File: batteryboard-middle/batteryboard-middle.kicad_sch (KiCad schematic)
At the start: 10 parts, among them J1 Conn_01x02, J2 Conn_01x02, J3 FLE-110-01-G-DV-A, J4 FLE-110-01-G-DV-A, J5 FTS-110-01-L-DV-A, J6 FTS-110-01-L-DV-A

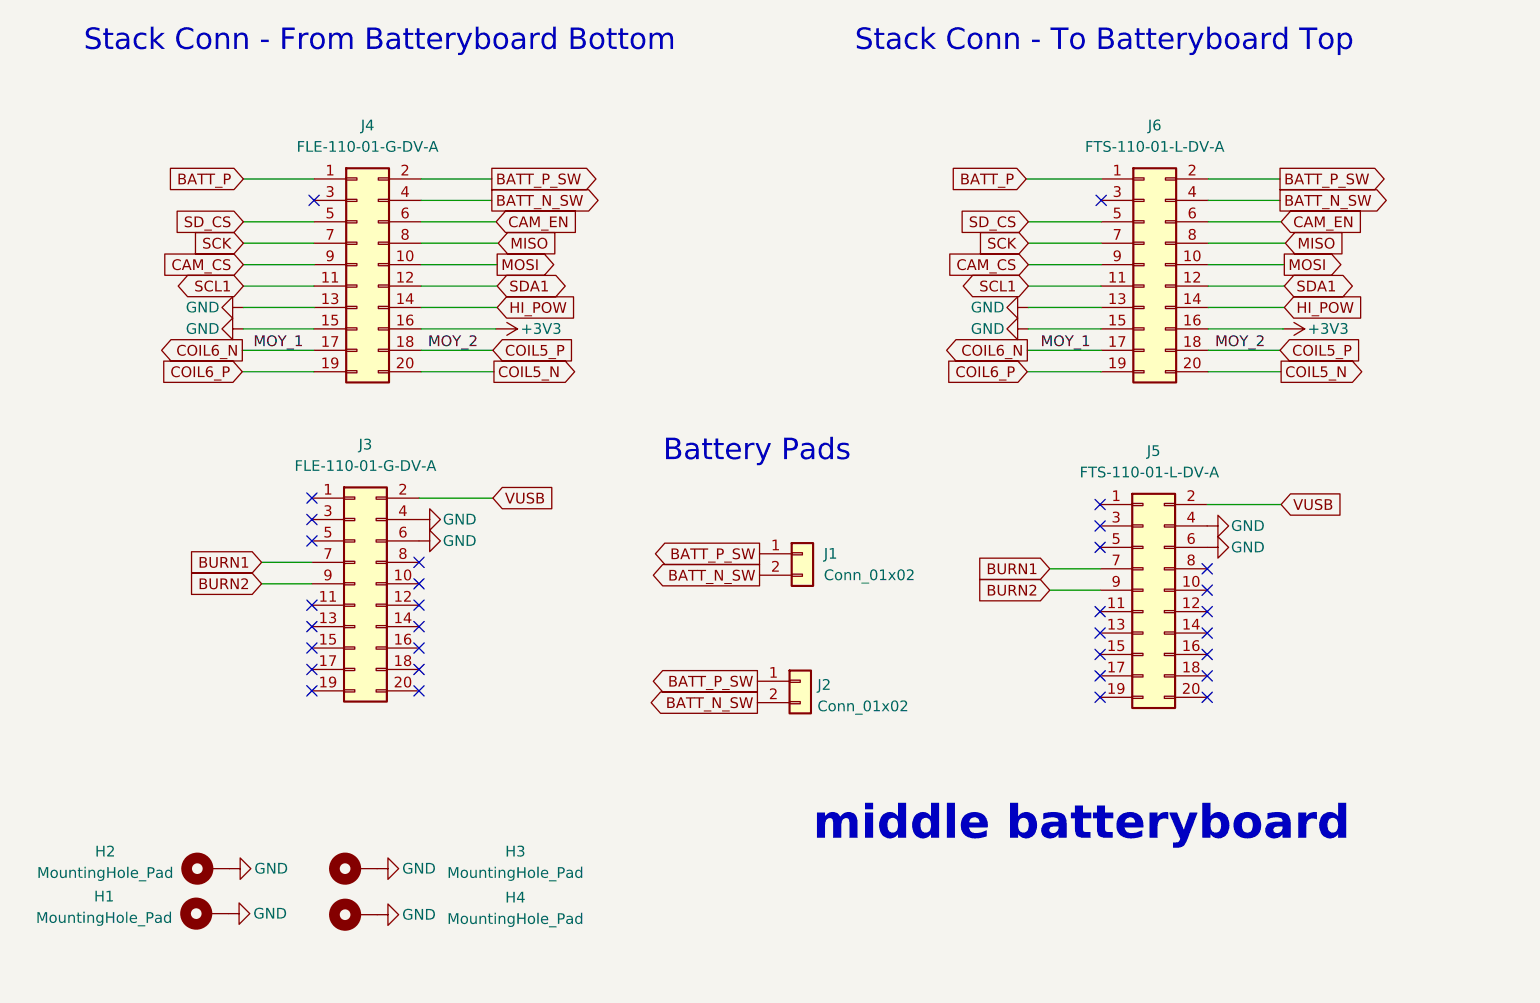
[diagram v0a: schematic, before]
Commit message: Fixed Broken Merge
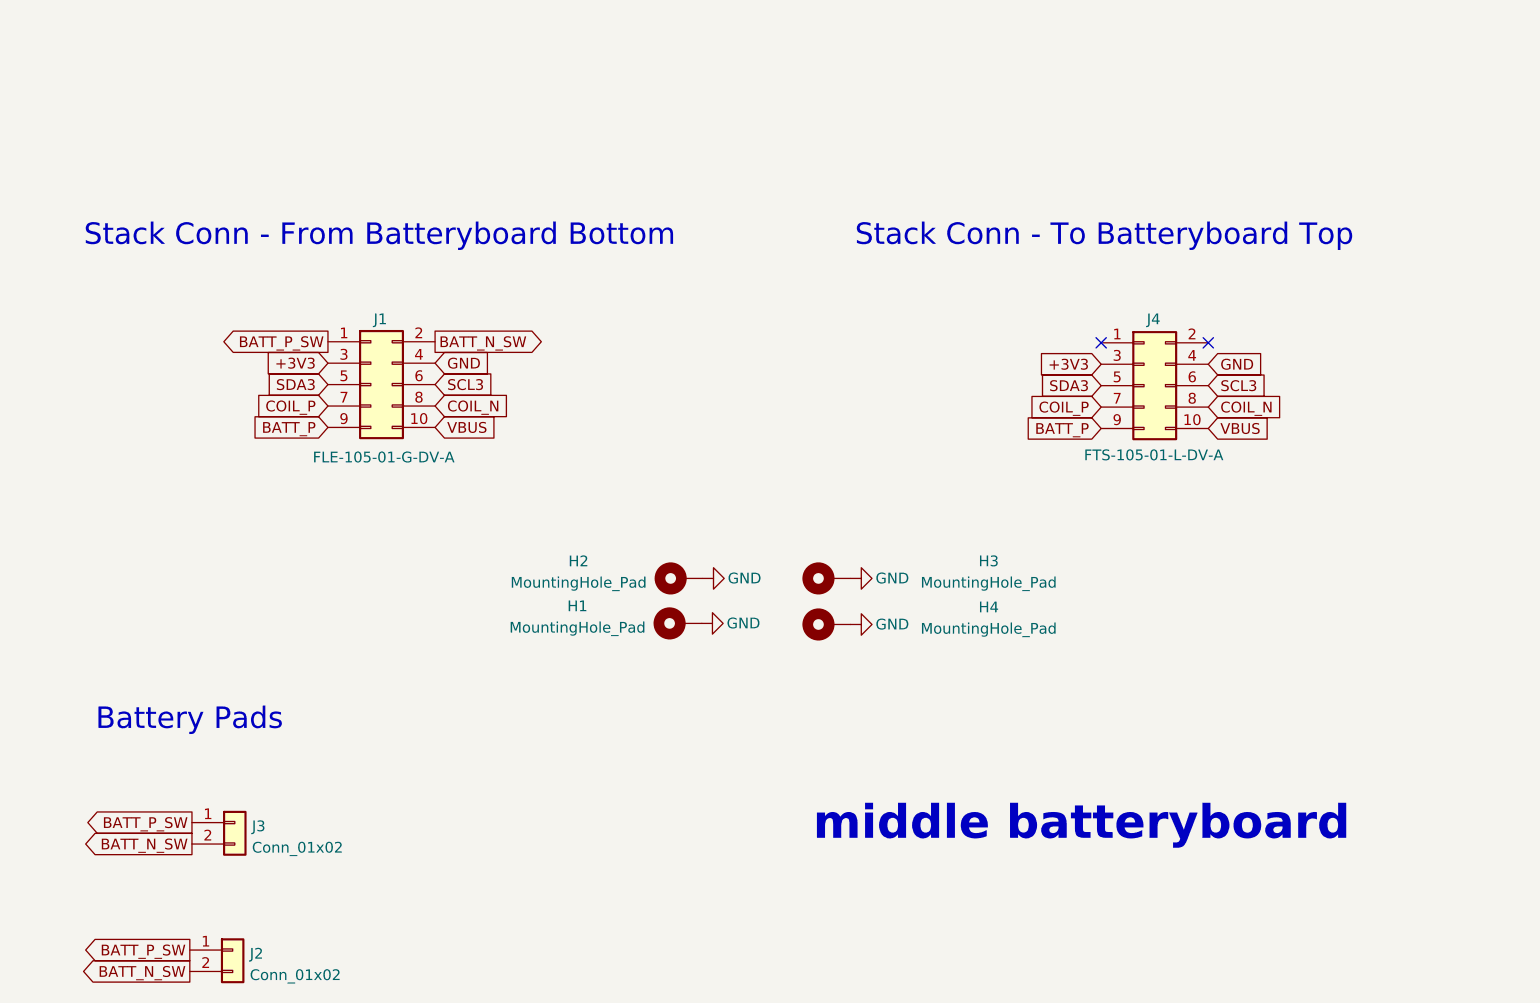
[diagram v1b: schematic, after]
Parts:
- removed J3, J4: FLE-110-01-G-DV-A, mainboard:SAMTEC_FLE-110-01-G-DV-A, symbol Connector_Generic:Conn_02x10_Odd_Even
- removed J5, J6: FTS-110-01-L-DV-A, batteryboard:SAMTEC-FTS-110-01-X-DV-A, symbol Connector_Generic:Conn_02x10_Odd_Even
- added J1: FLE-105-01-G-DV-A, batteryboard:SAMTEC_FLE-105-01-G-DV-A, symbol Connector_Generic:Conn_02x05_Odd_Even
- added J4: FTS-105-01-L-DV-A, batteryboard:FTS-105-XX-YY-DV-A, symbol Connector_Generic:Conn_02x05_Odd_Even
- renumbered J1 to J3
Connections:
- net +3V3: now also J1.3 (Pin_3), J4.3 (Pin_3)
- net BATT_N_SW: now also J1.2 (Pin_2)
- net BATT_P: now also J1.9 (Pin_9), J4.9 (Pin_9)
- net BATT_P_SW: now also J1.1 (Pin_1)
- net GND: now also J1.4 (Pin_4), J4.4 (Pin_4)
- new net COIL_N: J1.8 (Pin_8), J4.8 (Pin_8)
- new net COIL_P: J1.7 (Pin_7), J4.7 (Pin_7)
- new net SCL3: J1.6 (Pin_6), J4.6 (Pin_6)
- new net SDA3: J1.5 (Pin_5), J4.5 (Pin_5)
- new net VBUS: J1.10 (Pin_10), J4.10 (Pin_10)
- no-connect marks 32 -> 2
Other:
- moved on the sheet: H1, H2, H3, H4, J2, J3
